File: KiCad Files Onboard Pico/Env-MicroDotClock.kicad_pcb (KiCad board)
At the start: 2 copper layers, 94 x 80 mm, 378 parts, among them IC1 IS31FL3730-QFLS2-TR, IC2 IS31FL3730-QFLS2-TR, IC3 IS31FL3730-QFLS2-TR, IC4 IS31FL3730-QFLS2-TR, J1 1mm 1x3, J201 GT-USB-7051A, J203 Button, Q1 2SC1815, SW1 MX Keyboard Switch, SW2 MX Keyboard Switch, SW3 MX Keyboard Switch, SW4 MX Keyboard Switch, SW5 MX Keyboard Switch, U1 TCA9406DC, U201 TPS63001DRCR, U202 RP2040, U3 DS3231MZ, Y201 3225_4P 12MHz

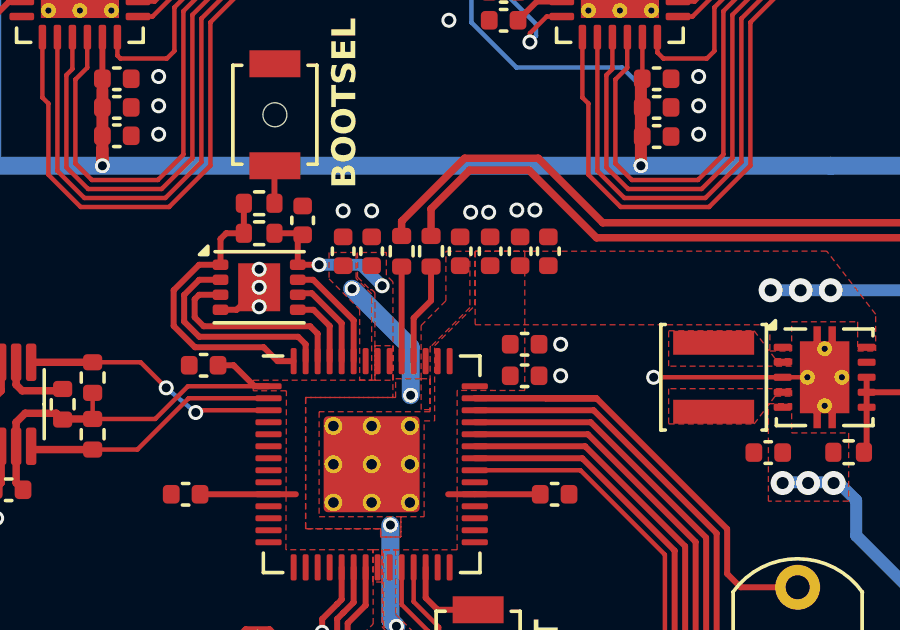
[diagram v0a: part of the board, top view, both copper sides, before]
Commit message: small corrections
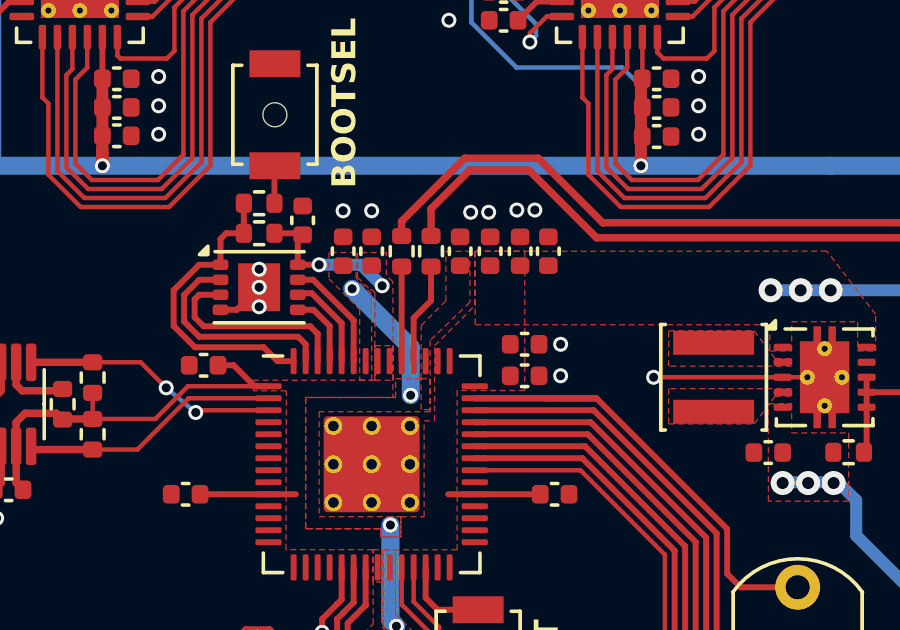
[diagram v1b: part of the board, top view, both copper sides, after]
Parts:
- R201, R202: value 5.1K 0402 -> 5K1 0402
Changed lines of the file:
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@@
 		(property ki_fp_filters "C_*")
 		(sheetname "Onboard Pico")
-		(sheetfile "untitled.kicad_sch")
+		(sheetfile "MCU.kicad_sch")
 		(attr smd)
 		(fp_line
@@
 		(property ki_fp_filters "R_*")
 		(sheetname "Onboard Pico")
-		(sheetfile "untitled.kicad_sch")
+		(sheetfile "MCU.kicad_sch")
 		(attr smd)
 		(fp_line
@@
 		(property ki_fp_filters "R_*")
 		(sheetname "Onboard Pico")
-		(sheetfile "untitled.kicad_sch")
+		(sheetfile "MCU.kicad_sch")
 		(attr smd)
 		(fp_line
@@
 		(property ki_fp_filters "C_*")
 		(sheetname "Onboard Pico")
-		(sheetfile "untitled.kicad_sch")
+		(sheetfile "MCU.kicad_sch")
 		(attr smd)
 		(fp_line
@@
 		(property ki_fp_filters "R_*")
 		(sheetname "Onboard Pico")
-		(sheetfile "untitled.kicad_sch")
+		(sheetfile "MCU.kicad_sch")
 		(attr smd)
 		(fp_line
@@
 		(property ki_fp_filters "C_*")
 		(sheetname "Onboard Pico")
-		(sheetfile "untitled.kicad_sch")
+		(sheetfile "MCU.kicad_sch")
 		(attr smd)
 		(fp_line
@@
 		(property ki_fp_filters "R_*")
 		(sheetname "Onboard Pico")
-		(sheetfile "untitled.kicad_sch")
+		(sheetfile "MCU.kicad_sch")
 		(attr smd)
 		(fp_line
@@
 		)
 		(sheetname "Onboard Pico")
-		(sheetfile "untitled.kicad_sch")
+		(sheetfile "MCU.kicad_sch")
 		(attr smd)
 		(fp_line
@@
 		(property ki_fp_filters "C_*")
 		(sheetname "Onboard Pico")
-		(sheetfile "untitled.kicad_sch")
+		(sheetfile "MCU.kicad_sch")
 		(attr smd)
 		(fp_line
@@
 		(property ki_fp_filters "C_*")
 		(sheetname "Onboard Pico")
-		(sheetfile "untitled.kicad_sch")
+		(sheetfile "MCU.kicad_sch")
 		(attr smd)
 		(fp_line
@@
 		(property ki_fp_filters "C_*")
 		(sheetname "Onboard Pico")
-		(sheetfile "untitled.kicad_sch")
+		(sheetfile "MCU.kicad_sch")
 		(attr smd)
 		(fp_line
@@
 		(property ki_fp_filters "Pin* Test*")
 		(sheetname "Onboard Pico")
-		(sheetfile "untitled.kicad_sch")
+		(sheetfile "MCU.kicad_sch")
 		(attr exclude_from_pos_files)
 		(fp_circle
@@
 		(property ki_fp_filters "Pin* Test*")
 		(sheetname "Onboard Pico")
-		(sheetfile "untitled.kicad_sch")
+		(sheetfile "MCU.kicad_sch")
 		(attr exclude_from_pos_files)
 		(fp_circle
@@
 		(property ki_fp_filters "Crystal*")
 		(sheetname "Onboard Pico")
-		(sheetfile "untitled.kicad_sch")
+		(sheetfile "MCU.kicad_sch")
 		(attr smd)
 		(fp_line
@@
 		(property ki_fp_filters "C_*")
 		(sheetname "Onboard Pico")
-		(sheetfile "untitled.kicad_sch")
+		(sheetfile "MCU.kicad_sch")
 		(attr smd)
 		(fp_line
@@
 		(property ki_fp_filters "Texas*DRC0010J*")
 		(sheetname "Onboard Pico")
-		(sheetfile "untitled.kicad_sch")
+		(sheetfile "MCU.kicad_sch")
 		(attr smd)
 		(fp_line
@@
 		(property ki_fp_filters "C_*")
 		(sheetname "Onboard Pico")
-		(sheetfile "untitled.kicad_sch")
+		(sheetfile "MCU.kicad_sch")
 		(attr smd)
 		(fp_line
@@
 		)
 		(sheetname "Onboard Pico")
-		(sheetfile "untitled.kicad_sch")
+		(sheetfile "MCU.kicad_sch")
 		(attr smd)
 		(fp_line
@@
 		(property ki_fp_filters "C_*")
 		(sheetname "Onboard Pico")
-		(sheetfile "untitled.kicad_sch")
+		(sheetfile "MCU.kicad_sch")
 		(attr smd)
 		(fp_line
@@
 		(property ki_fp_filters "Choke_* *Coil* Inductor_* L_*")
 		(sheetname "Onboard Pico")
-		(sheetfile "untitled.kicad_sch")
+		(sheetfile "MCU.kicad_sch")
 		(attr smd)
 		(fp_line
@@
 		(property ki_fp_filters "C_*")
 		(sheetname "Onboard Pico")
-		(sheetfile "untitled.kicad_sch")
+		(sheetfile "MCU.kicad_sch")
 		(attr smd)
 		(fp_line
@@
 		(property ki_fp_filters "C_*")
 		(sheetname "Onboard Pico")
-		(sheetfile "untitled.kicad_sch")
+		(sheetfile "MCU.kicad_sch")
 		(attr smd)
 		(fp_line
@@
 		(property ki_fp_filters "C_*")
 		(sheetname "Onboard Pico")
-		(sheetfile "untitled.kicad_sch")
+		(sheetfile "MCU.kicad_sch")
 		(attr smd)
 		(fp_line
@@
 		(property ki_fp_filters "C_*")
 		(sheetname "Onboard Pico")
-		(sheetfile "untitled.kicad_sch")
+		(sheetfile "MCU.kicad_sch")
 		(attr smd)
 		(fp_line
@@
 		(property ki_fp_filters "R_*")
 		(sheetname "Onboard Pico")
-		(sheetfile "untitled.kicad_sch")
+		(sheetfile "MCU.kicad_sch")
 		(attr smd)
 		(fp_line
@@
 		(property ki_fp_filters "C_*")
 		(sheetname "Onboard Pico")
-		(sheetfile "untitled.kicad_sch")
+		(sheetfile "MCU.kicad_sch")
 		(attr smd)
 		(fp_line
@@
 		(property ki_fp_filters "R_*")
 		(sheetname "Onboard Pico")
-		(sheetfile "untitled.kicad_sch")
+		(sheetfile "MCU.kicad_sch")
 		(attr smd)
 		(fp_line
@@
 		(property ki_fp_filters "C_*")
 		(sheetname "Onboard Pico")
-		(sheetfile "untitled.kicad_sch")
+		(sheetfile "MCU.kicad_sch")
 		(attr smd)
 		(fp_line
@@
 		(property ki_fp_filters "WSON*1EP*6x5mm*P1.27mm*")
 		(sheetname "Onboard Pico")
-		(sheetfile "untitled.kicad_sch")
+		(sheetfile "MCU.kicad_sch")
 		(attr smd)
 		(fp_line
@@
 		(property ki_fp_filters "C_*")
 		(sheetname "Onboard Pico")
-		(sheetfile "untitled.kicad_sch")
+		(sheetfile "MCU.kicad_sch")
 		(attr smd)
 		(fp_line
@@
 		(property ki_fp_filters "C_*")
 		(sheetname "Onboard Pico")
-		(sheetfile "untitled.kicad_sch")
+		(sheetfile "MCU.kicad_sch")
 		(attr smd)
 		(fp_line
@@
 		)
 		(sheetname "Onboard Pico")
-		(sheetfile "untitled.kicad_sch")
+		(sheetfile "MCU.kicad_sch")
 		(attr smd)
 		(fp_line
@@
 		(property ki_fp_filters "C_*")
 		(sheetname "Onboard Pico")
-		(sheetfile "untitled.kicad_sch")
+		(sheetfile "MCU.kicad_sch")
 		(attr smd)
 		(fp_line
@@
 			)
 		)
-		(property "Value" "5.1K 0402"
+		(property "Value" "5K1 0402"
 			(at 0 -1.17 90)
 			(layer "B.Fab")
@@
 		(property ki_fp_filters "R_*")
 		(sheetname "Onboard Pico")
-		(sheetfile "untitled.kicad_sch")
+		(sheetfile "MCU.kicad_sch")
 		(attr smd)
 		(fp_line
@@
 		(property ki_fp_filters "USB*C*Receptacle*")
 		(sheetname "Onboard Pico")
-		(sheetfile "untitled.kicad_sch")
+		(sheetfile "MCU.kicad_sch")
 		(attr smd)
 		(fp_line
@@
 		(property ki_fp_filters "TO-???* *_Diode_* *SingleDiode* D_*")
 		(sheetname "Onboard Pico")
-		(sheetfile "untitled.kicad_sch")
+		(sheetfile "MCU.kicad_sch")
 		(attr smd)
 		(fp_line
@@
 			)
 		)
-		(property "Value" "5.1K 0402"
+		(property "Value" "5K1 0402"
 			(at 0 -1.17 90)
 			(layer "B.Fab")
@@
 		(property ki_fp_filters "R_*")
 		(sheetname "Onboard Pico")
-		(sheetfile "untitled.kicad_sch")
+		(sheetfile "MCU.kicad_sch")
 		(attr smd)
 		(fp_line
@@
 		(polygon
 			(pts
-				(xy 71.775 55.9) (xy 71.775 57.775) (xy 70.476385 59.073615) (xy 70.448839 59.073615) (xy 70.448839 60.148839)
-				(xy 70.448839 61.178615) (xy 70.150224 61.18) (xy 70.148839 60.148615) (xy 70.148839 58.376161)
-				(xy 70.975 57.55) (xy 70.975 55.9)
+				(xy 71.775 55.9) (xy 71.775 57.6) (xy 70.448839 58.873615) (xy 70.448839 60.148839) (xy 70.448839 61.178615)
+				(xy 70.150224 61.18) (xy 70.148839 60.148615) (xy 70.148839 58.376161) (xy 70.975 57.55) (xy 70.975 55.9)
 			)
 		)
